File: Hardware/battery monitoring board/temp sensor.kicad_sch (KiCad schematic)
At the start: 11 parts, among them J2 Conn_01x02, U1 MAX31855KASA

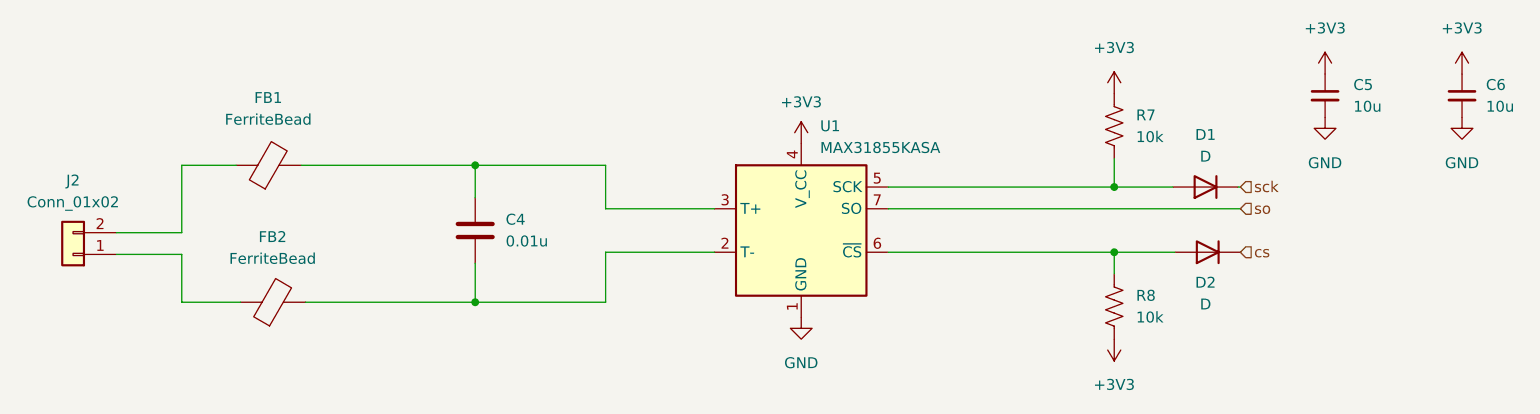
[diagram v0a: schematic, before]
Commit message: Updated reference labels
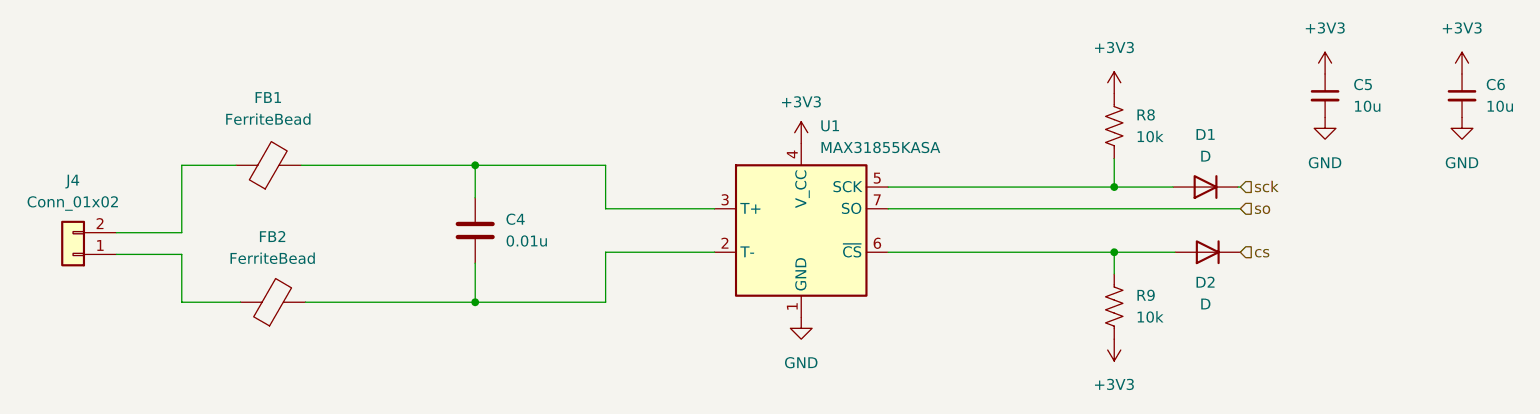
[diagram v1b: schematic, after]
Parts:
- renumbered J2 to J4, R7 to R8, R8 to R9
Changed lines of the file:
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@@
   (symbol (lib_id "PCM_4ms_Power-symbol:GND") (at 141.224 108.966 0) (unit 1)
     (in_bom yes) (on_board yes) (dnp no) (fields_autoplaced)
-    (property "Reference" "#PWR08" (at 141.224 115.316 0)
+    (property "Reference" "#PWR012" (at 141.224 115.316 0)
       (effects (font (size 1.27 1.27)) hide)
     )
@@
       (project "battery monitoring board"
         (path "/bf623d80-ca5a-491f-9daa-4dffbeba5279/5ec2dbdf-a276-4d4c-99fc-008475c1e770"
-          (reference "#PWR08") (unit 1)
+          (reference "#PWR012") (unit 1)
         )
       )
@@
   (symbol (lib_id "power:+3V3") (at 202.438 80.518 0) (unit 1)
     (in_bom yes) (on_board yes) (dnp no) (fields_autoplaced)
-    (property "Reference" "#PWR011" (at 202.438 84.328 0)
+    (property "Reference" "#PWR015" (at 202.438 84.328 0)
       (effects (font (size 1.27 1.27)) hide)
     )
@@
       (project "battery monitoring board"
         (path "/bf623d80-ca5a-491f-9daa-4dffbeba5279/5ec2dbdf-a276-4d4c-99fc-008475c1e770"
-          (reference "#PWR011") (unit 1)
+          (reference "#PWR015") (unit 1)
         )
       )
@@
   (symbol (lib_id "Device:R_US") (at 177.8 86.614 0) (unit 1)
     (in_bom yes) (on_board yes) (dnp no) (fields_autoplaced)
-    (property "Reference" "R7" (at 180.34 85.344 0)
+    (property "Reference" "R8" (at 180.34 85.344 0)
       (effects (font (size 1.27 1.27)) (justify left))
     )
@@
       (project "battery monitoring board"
         (path "/bf623d80-ca5a-491f-9daa-4dffbeba5279/5ec2dbdf-a276-4d4c-99fc-008475c1e770"
-          (reference "R7") (unit 1)
+          (reference "R8") (unit 1)
         )
       )
@@
   (symbol (lib_id "Device:R_US") (at 177.8 107.696 0) (unit 1)
     (in_bom yes) (on_board yes) (dnp no) (fields_autoplaced)
-    (property "Reference" "R8" (at 180.34 106.426 0)
+    (property "Reference" "R9" (at 180.34 106.426 0)
       (effects (font (size 1.27 1.27)) (justify left))
     )
@@
       (project "battery monitoring board"
         (path "/bf623d80-ca5a-491f-9daa-4dffbeba5279/5ec2dbdf-a276-4d4c-99fc-008475c1e770"
-          (reference "R8") (unit 1)
+          (reference "R9") (unit 1)
         )
       )
@@
   (symbol (lib_id "power:+3V3") (at 177.8 111.506 180) (unit 1)
     (in_bom yes) (on_board yes) (dnp no) (fields_autoplaced)
-    (property "Reference" "#PWR010" (at 177.8 107.696 0)
+    (property "Reference" "#PWR014" (at 177.8 107.696 0)
       (effects (font (size 1.27 1.27)) hide)
     )
@@
       (project "battery monitoring board"
         (path "/bf623d80-ca5a-491f-9daa-4dffbeba5279/5ec2dbdf-a276-4d4c-99fc-008475c1e770"
-          (reference "#PWR010") (unit 1)
+          (reference "#PWR014") (unit 1)
         )
       )
@@
   (symbol (lib_id "PCM_4ms_Power-symbol:GND") (at 202.438 85.598 0) (unit 1)
     (in_bom yes) (on_board yes) (dnp no) (fields_autoplaced)
-    (property "Reference" "#PWR012" (at 202.438 91.948 0)
+    (property "Reference" "#PWR016" (at 202.438 91.948 0)
       (effects (font (size 1.27 1.27)) hide)
     )
@@
       (project "battery monitoring board"
         (path "/bf623d80-ca5a-491f-9daa-4dffbeba5279/5ec2dbdf-a276-4d4c-99fc-008475c1e770"
-          (reference "#PWR012") (unit 1)
+          (reference "#PWR016") (unit 1)
         )
       )
@@
   (symbol (lib_id "PCM_4ms_Power-symbol:GND") (at 218.44 85.598 0) (unit 1)
     (in_bom yes) (on_board yes) (dnp no) (fields_autoplaced)
-    (property "Reference" "#PWR014" (at 218.44 91.948 0)
+    (property "Reference" "#PWR018" (at 218.44 91.948 0)
       (effects (font (size 1.27 1.27)) hide)
     )
@@
       (project "battery monitoring board"
         (path "/bf623d80-ca5a-491f-9daa-4dffbeba5279/5ec2dbdf-a276-4d4c-99fc-008475c1e770"
-          (reference "#PWR014") (unit 1)
+          (reference "#PWR018") (unit 1)
         )
       )
@@
   (symbol (lib_id "PCM_4ms_Connector:Conn_01x02") (at 56.134 101.6 180) (unit 1)
     (in_bom yes) (on_board yes) (dnp no) (fields_autoplaced)
-    (property "Reference" "J2" (at 56.134 92.964 0)
+    (property "Reference" "J4" (at 56.134 92.964 0)
       (effects (font (size 1.27 1.27)))
     )
@@
       (project "battery monitoring board"
         (path "/bf623d80-ca5a-491f-9daa-4dffbeba5279/5ec2dbdf-a276-4d4c-99fc-008475c1e770"
-          (reference "J2") (unit 1)
+          (reference "J4") (unit 1)
         )
       )
@@
   (symbol (lib_id "power:+3V3") (at 218.44 80.518 0) (unit 1)
     (in_bom yes) (on_board yes) (dnp no) (fields_autoplaced)
-    (property "Reference" "#PWR013" (at 218.44 84.328 0)
+    (property "Reference" "#PWR017" (at 218.44 84.328 0)
       (effects (font (size 1.27 1.27)) hide)
     )
@@
       (project "battery monitoring board"
         (path "/bf623d80-ca5a-491f-9daa-4dffbeba5279/5ec2dbdf-a276-4d4c-99fc-008475c1e770"
+          (reference "#PWR017") (unit 1)
+        )
+      )
+    )
+  )
+  (symbol (lib_id "power:+3V3") (at 141.224 88.646 0) (unit 1)
+    (in_bom yes) (on_board yes) (dnp no) (fields_autoplaced)
+    (property "Reference" "#PWR011" (at 141.224 92.456 0)
+      (effects (font (size 1.27 1.27)) hide)
+    )
+    (property "Value" "+3V3" (at 141.224 83.82 0)
+      (effects (font (size 1.27 1.27)))
+    )
+    (property "Footprint" "" (at 141.224 88.646 0)
+      (effects (font (size 1.27 1.27)) hide)
+    )
+    (property "Datasheet" "" (at 141.224 88.646 0)
+      (effects (font (size 1.27 1.27)) hide)
+    )
+    (pin "1")
+    (instances
+      (project "battery monitoring board"
+        (path "/bf623d80-ca5a-491f-9daa-4dffbeba5279/5ec2dbdf-a276-4d4c-99fc-008475c1e770"
+          (reference "#PWR011") (unit 1)
+        )
+      )
+    )
+  )
+  (symbol (lib_id "power:+3V3") (at 177.8 82.804 0) (unit 1)
+    (in_bom yes) (on_board yes) (dnp no) (fields_autoplaced)
+    (property "Reference" "#PWR013" (at 177.8 86.614 0)
+      (effects (font (size 1.27 1.27)) hide)
+    )
+    (property "Value" "+3V3" (at 177.8 77.47 0)
+      (effects (font (size 1.27 1.27)))
+    )
+    (property "Footprint" "" (at 177.8 82.804 0)
+      (effects (font (size 1.27 1.27)) hide)
+    )
+    (property "Datasheet" "" (at 177.8 82.804 0)
+      (effects (font (size 1.27 1.27)) hide)
+    )
+    (pin "1")
+    (instances
+      (project "battery monitoring board"
+        (path "/bf623d80-ca5a-491f-9daa-4dffbeba5279/5ec2dbdf-a276-4d4c-99fc-008475c1e770"
           (reference "#PWR013") (unit 1)
         )
       )
-    )
-  )
-  (symbol (lib_id "power:+3V3") (at 141.224 88.646 0) (unit 1)
-    (in_bom yes) (on_board yes) (dnp no) (fields_autoplaced)
-    (property "Reference" "#PWR07" (at 141.224 92.456 0)
-      (effects (font (size 1.27 1.27)) hide)
-    )
-    (property "Value" "+3V3" (at 141.224 83.82 0)
-      (effects (font (size 1.27 1.27)))
-    )
-    (property "Footprint" "" (at 141.224 88.646 0)
-      (effects (font (size 1.27 1.27)) hide)
-    )
-    (property "Datasheet" "" (at 141.224 88.646 0)
-      (effects (font (size 1.27 1.27)) hide)
-    )
-    (pin "1")
-    (instances
-      (project "battery monitoring board"
-        (path "/bf623d80-ca5a-491f-9daa-4dffbeba5279/5ec2dbdf-a276-4d4c-99fc-008475c1e770"
-          (reference "#PWR07") (unit 1)
-        )
-      )
-    )
-  )
-  (symbol (lib_id "power:+3V3") (at 177.8 82.804 0) (unit 1)
-    (in_bom yes) (on_board yes) (dnp no) (fields_autoplaced)
-    (property "Reference" "#PWR09" (at 177.8 86.614 0)
-      (effects (font (size 1.27 1.27)) hide)
-    )
-    (property "Value" "+3V3" (at 177.8 77.47 0)
-      (effects (font (size 1.27 1.27)))
-    )
-    (property "Footprint" "" (at 177.8 82.804 0)
-      (effects (font (size 1.27 1.27)) hide)
-    )
-    (property "Datasheet" "" (at 177.8 82.804 0)
-      (effects (font (size 1.27 1.27)) hide)
-    )
-    (pin "1")
-    (instances
-      (project "battery monitoring board"
-        (path "/bf623d80-ca5a-491f-9daa-4dffbeba5279/5ec2dbdf-a276-4d4c-99fc-008475c1e770"
-          (reference "#PWR09") (unit 1)
-        )
-      )

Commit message: Revert "Updated reference labels"
This reverts commit 7ccd23260c988ead49c0bcfa936e50f6d09a7000.
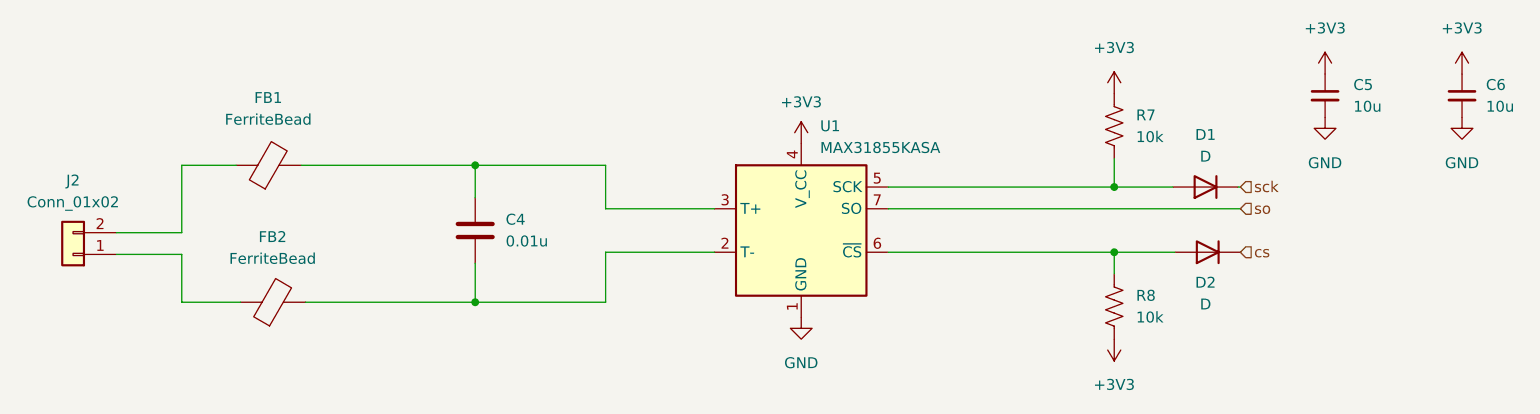
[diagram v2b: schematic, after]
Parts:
- renumbered J4 to J2, R8 to R7, R9 to R8
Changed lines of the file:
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@@
   (symbol (lib_id "PCM_4ms_Power-symbol:GND") (at 141.224 108.966 0) (unit 1)
     (in_bom yes) (on_board yes) (dnp no) (fields_autoplaced)
-    (property "Reference" "#PWR012" (at 141.224 115.316 0)
+    (property "Reference" "#PWR08" (at 141.224 115.316 0)
       (effects (font (size 1.27 1.27)) hide)
     )
@@
       (project "battery monitoring board"
         (path "/bf623d80-ca5a-491f-9daa-4dffbeba5279/5ec2dbdf-a276-4d4c-99fc-008475c1e770"
-          (reference "#PWR012") (unit 1)
+          (reference "#PWR08") (unit 1)
         )
       )
@@
   (symbol (lib_id "power:+3V3") (at 202.438 80.518 0) (unit 1)
     (in_bom yes) (on_board yes) (dnp no) (fields_autoplaced)
-    (property "Reference" "#PWR015" (at 202.438 84.328 0)
+    (property "Reference" "#PWR011" (at 202.438 84.328 0)
       (effects (font (size 1.27 1.27)) hide)
     )
@@
       (project "battery monitoring board"
         (path "/bf623d80-ca5a-491f-9daa-4dffbeba5279/5ec2dbdf-a276-4d4c-99fc-008475c1e770"
-          (reference "#PWR015") (unit 1)
+          (reference "#PWR011") (unit 1)
         )
       )
@@
   (symbol (lib_id "Device:R_US") (at 177.8 86.614 0) (unit 1)
     (in_bom yes) (on_board yes) (dnp no) (fields_autoplaced)
-    (property "Reference" "R8" (at 180.34 85.344 0)
+    (property "Reference" "R7" (at 180.34 85.344 0)
       (effects (font (size 1.27 1.27)) (justify left))
     )
@@
       (project "battery monitoring board"
         (path "/bf623d80-ca5a-491f-9daa-4dffbeba5279/5ec2dbdf-a276-4d4c-99fc-008475c1e770"
+          (reference "R7") (unit 1)
+        )
+      )
+    )
+  )
+  (symbol (lib_id "Device:R_US") (at 177.8 107.696 0) (unit 1)
+    (in_bom yes) (on_board yes) (dnp no) (fields_autoplaced)
+    (property "Reference" "R8" (at 180.34 106.426 0)
+      (effects (font (size 1.27 1.27)) (justify left))
+    )
+    (property "Value" "10k" (at 180.34 108.966 0)
+      (effects (font (size 1.27 1.27)) (justify left))
+    )
+    (property "Footprint" "" (at 178.816 107.95 90)
+      (effects (font (size 1.27 1.27)) hide)
+    )
+    (property "Datasheet" "~" (at 177.8 107.696 0)
+      (effects (font (size 1.27 1.27)) hide)
+    )
+    (pin "1")
+    (pin "2")
+    (instances
+      (project "battery monitoring board"
+        (path "/bf623d80-ca5a-491f-9daa-4dffbeba5279/5ec2dbdf-a276-4d4c-99fc-008475c1e770"
           (reference "R8") (unit 1)
         )
@@
     )
   )
-  (symbol (lib_id "Device:R_US") (at 177.8 107.696 0) (unit 1)
-    (in_bom yes) (on_board yes) (dnp no) (fields_autoplaced)
-    (property "Reference" "R9" (at 180.34 106.426 0)
-      (effects (font (size 1.27 1.27)) (justify left))
-    )
-    (property "Value" "10k" (at 180.34 108.966 0)
-      (effects (font (size 1.27 1.27)) (justify left))
-    )
-    (property "Footprint" "" (at 178.816 107.95 90)
-      (effects (font (size 1.27 1.27)) hide)
-    )
-    (property "Datasheet" "~" (at 177.8 107.696 0)
-      (effects (font (size 1.27 1.27)) hide)
-    )
-    (pin "1")
-    (pin "2")
-    (instances
-      (project "battery monitoring board"
-        (path "/bf623d80-ca5a-491f-9daa-4dffbeba5279/5ec2dbdf-a276-4d4c-99fc-008475c1e770"
-          (reference "R9") (unit 1)
-        )
-      )
-    )
-  )
   (symbol (lib_id "Device:C") (at 103.124 98.806 0) (unit 1)
     (in_bom yes) (on_board yes) (dnp no) (fields_autoplaced)
@@
   (symbol (lib_id "power:+3V3") (at 177.8 111.506 180) (unit 1)
     (in_bom yes) (on_board yes) (dnp no) (fields_autoplaced)
-    (property "Reference" "#PWR014" (at 177.8 107.696 0)
+    (property "Reference" "#PWR010" (at 177.8 107.696 0)
       (effects (font (size 1.27 1.27)) hide)
     )
@@
       (project "battery monitoring board"
         (path "/bf623d80-ca5a-491f-9daa-4dffbeba5279/5ec2dbdf-a276-4d4c-99fc-008475c1e770"
-          (reference "#PWR014") (unit 1)
+          (reference "#PWR010") (unit 1)
         )
       )
@@
   (symbol (lib_id "PCM_4ms_Power-symbol:GND") (at 202.438 85.598 0) (unit 1)
     (in_bom yes) (on_board yes) (dnp no) (fields_autoplaced)
-    (property "Reference" "#PWR016" (at 202.438 91.948 0)
+    (property "Reference" "#PWR012" (at 202.438 91.948 0)
       (effects (font (size 1.27 1.27)) hide)
     )
@@
       (project "battery monitoring board"
         (path "/bf623d80-ca5a-491f-9daa-4dffbeba5279/5ec2dbdf-a276-4d4c-99fc-008475c1e770"
-          (reference "#PWR016") (unit 1)
+          (reference "#PWR012") (unit 1)
         )
       )
@@
   (symbol (lib_id "PCM_4ms_Power-symbol:GND") (at 218.44 85.598 0) (unit 1)
     (in_bom yes) (on_board yes) (dnp no) (fields_autoplaced)
-    (property "Reference" "#PWR018" (at 218.44 91.948 0)
+    (property "Reference" "#PWR014" (at 218.44 91.948 0)
       (effects (font (size 1.27 1.27)) hide)
     )
@@
       (project "battery monitoring board"
         (path "/bf623d80-ca5a-491f-9daa-4dffbeba5279/5ec2dbdf-a276-4d4c-99fc-008475c1e770"
-          (reference "#PWR018") (unit 1)
+          (reference "#PWR014") (unit 1)
         )
       )
@@
   (symbol (lib_id "PCM_4ms_Connector:Conn_01x02") (at 56.134 101.6 180) (unit 1)
     (in_bom yes) (on_board yes) (dnp no) (fields_autoplaced)
-    (property "Reference" "J4" (at 56.134 92.964 0)
+    (property "Reference" "J2" (at 56.134 92.964 0)
       (effects (font (size 1.27 1.27)))
     )
@@
       (project "battery monitoring board"
         (path "/bf623d80-ca5a-491f-9daa-4dffbeba5279/5ec2dbdf-a276-4d4c-99fc-008475c1e770"
-          (reference "J4") (unit 1)
+          (reference "J2") (unit 1)
         )
       )
@@
   (symbol (lib_id "power:+3V3") (at 218.44 80.518 0) (unit 1)
     (in_bom yes) (on_board yes) (dnp no) (fields_autoplaced)
-    (property "Reference" "#PWR017" (at 218.44 84.328 0)
+    (property "Reference" "#PWR013" (at 218.44 84.328 0)
       (effects (font (size 1.27 1.27)) hide)
     )
@@
       (project "battery monitoring board"
         (path "/bf623d80-ca5a-491f-9daa-4dffbeba5279/5ec2dbdf-a276-4d4c-99fc-008475c1e770"
-          (reference "#PWR017") (unit 1)
+          (reference "#PWR013") (unit 1)
         )
       )
@@
   (symbol (lib_id "power:+3V3") (at 141.224 88.646 0) (unit 1)
     (in_bom yes) (on_board yes) (dnp no) (fields_autoplaced)
-    (property "Reference" "#PWR011" (at 141.224 92.456 0)
+    (property "Reference" "#PWR07" (at 141.224 92.456 0)
       (effects (font (size 1.27 1.27)) hide)
     )
@@
       (project "battery monitoring board"
         (path "/bf623d80-ca5a-491f-9daa-4dffbeba5279/5ec2dbdf-a276-4d4c-99fc-008475c1e770"
-          (reference "#PWR011") (unit 1)
+          (reference "#PWR07") (unit 1)
         )
       )
@@
   (symbol (lib_id "power:+3V3") (at 177.8 82.804 0) (unit 1)
     (in_bom yes) (on_board yes) (dnp no) (fields_autoplaced)
-    (property "Reference" "#PWR013" (at 177.8 86.614 0)
+    (property "Reference" "#PWR09" (at 177.8 86.614 0)
       (effects (font (size 1.27 1.27)) hide)
     )
@@
       (project "battery monitoring board"
         (path "/bf623d80-ca5a-491f-9daa-4dffbeba5279/5ec2dbdf-a276-4d4c-99fc-008475c1e770"
-          (reference "#PWR013") (unit 1)
-        )
-      )
+          (reference "#PWR09") (unit 1)
+        )
+      )
